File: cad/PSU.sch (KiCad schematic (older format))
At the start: 15 parts, among them J1 Input, J2 INA219 breakout, J3 Output, J4 WWG-A, J5 WWG-B, Q1 LM317T, U1 LM7805_TO220, U3 X9C103P

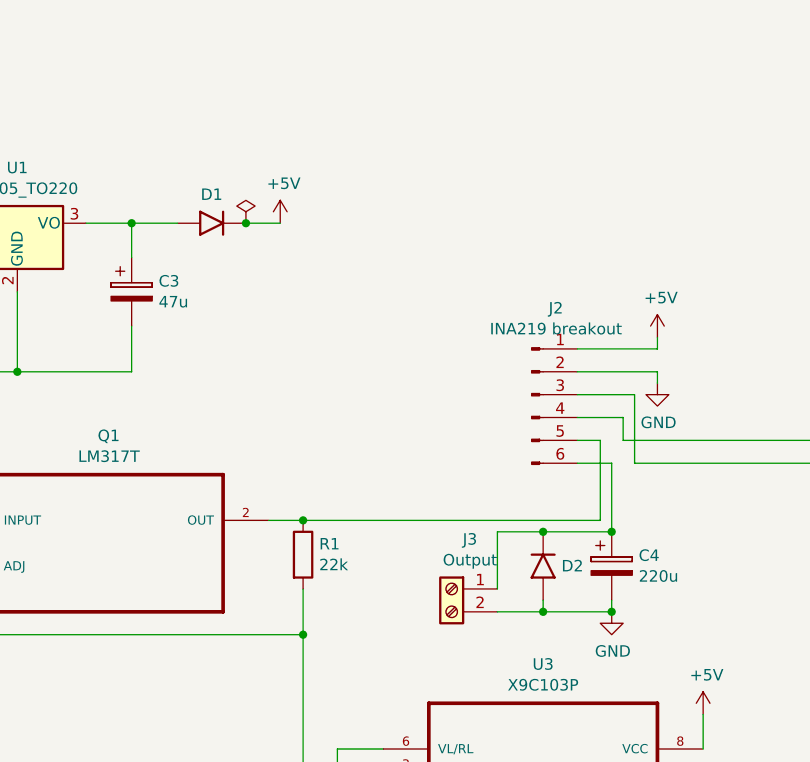
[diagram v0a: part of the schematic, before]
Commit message: first layout
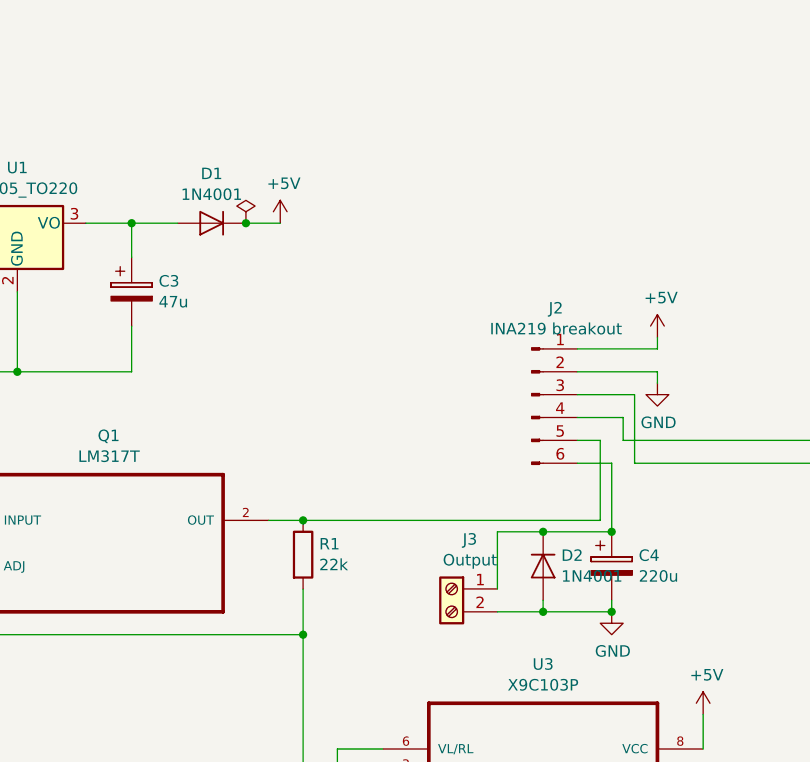
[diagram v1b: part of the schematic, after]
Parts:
- removed D1, D2: 1N4001, Diode_THT:D_A-405_P10.16mm_Horizontal, symbol 1N4001:1N4001
- added D1, D2: 1N4001, Diode_THT:D_DO-41_SOD81_P10.16mm_Horizontal, symbol Diode:1N4001
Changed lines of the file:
@@
 Wire Wire Line
 	7150 3200 7200 3200
-$Comp
-L 1N4001:1N4001 D1
-U 1 1 5CE165D2
-P 4200 2650
-F 0 "D1" H 4250 2775 50  0000 C CNN
-F 1 "1N4001" H 4200 2650 50  0001 L BNN
-F 2 "Diode_THT:D_A-405_P10.16mm_Horizontal" H 4200 2650 50  0001 L BNN
-F 3 "ON Semiconductor" H 4200 2650 50  0001 L BNN
-F 4 "None" H 4200 2650 50  0001 L BNN "Field4"
-F 5 "DO-41 ON Semiconductor" H 4200 2650 50  0001 L BNN "Field5"
-F 6 "Unavailable" H 4200 2650 50  0001 L BNN "Field6"
-F 7 "1N4001" H 4200 2650 50  0001 L BNN "Field7"
-F 8 "Diode, Standard, 1A, 50V" H 4200 2650 50  0001 L BNN "Field8"
-	1    4200 2650
-	1    0    0    -1
-$EndComp
 Wire Wire Line
 	3900 2650 4100 2650
@@
 Wire Wire Line
 	5500 4000 5500 4250
-Wire Wire Line
-	5500 4000 5700 4000
 Wire Wire Line
 	5500 4350 5700 4350
@@
 $EndComp
 Connection ~ 6000 4000
-$Comp
-L 1N4001:1N4001 D2
-U 1 1 5CE1E838
-P 5700 4200
-F 0 "D2" V 5750 4120 50  0000 R CNN
-F 1 "1N4001" H 5700 4200 50  0001 L BNN
-F 2 "Diode_THT:D_A-405_P10.16mm_Horizontal" H 5700 4200 50  0001 L BNN
-F 3 "ON Semiconductor" H 5700 4200 50  0001 L BNN
-F 4 "None" H 5700 4200 50  0001 L BNN "Field4"
-F 5 "DO-41 ON Semiconductor" H 5700 4200 50  0001 L BNN "Field5"
-F 6 "Unavailable" H 5700 4200 50  0001 L BNN "Field6"
-F 7 "1N4001" H 5700 4200 50  0001 L BNN "Field7"
-F 8 "Diode, Standard, 1A, 50V" H 5700 4200 50  0001 L BNN "Field8"
-	1    5700 4200
-	0    -1   -1   0
-$EndComp
-Connection ~ 5700 4000
-Wire Wire Line
-	5700 4000 6000 4000
 Wire Wire Line
 	6000 4300 6000 4350
@@
 	1    0    0    -1
 $EndComp
-Connection ~ 4400 2650
 Wire Wire Line
 	2500 4150 2650 4150
@@
 NoConn ~ 7200 3500
 NoConn ~ 5000 5050
+$Comp
+L Diode:1N4001 D1
+U 1 1 5CE7B69A
+P 4250 2650
+F 0 "D1" H 4250 2434 50  0000 C CNN
+F 1 "1N4001" H 4250 2525 50  0000 C CNN
+F 2 "Diode_THT:D_DO-41_SOD81_P10.16mm_Horizontal" H 4250 2475 50  0001 C CNN
+F 3 "http://www.vishay.com/docs/88503/1n4001.pdf" H 4250 2650 50  0001 C CNN
+	1    4250 2650
+	-1   0    0    1
+$EndComp
+Connection ~ 4400 2650
+Wire Wire Line
+	5500 4000 5700 4000
+$Comp
+L Diode:1N4001 D2
+U 1 1 5CE80A0F
+P 5700 4150
+F 0 "D2" V 5654 4229 50  0000 L CNN
+F 1 "1N4001" V 5745 4229 50  0000 L CNN
+F 2 "Diode_THT:D_DO-41_SOD81_P10.16mm_Horizontal" H 5700 3975 50  0001 C CNN
+F 3 "http://www.vishay.com/docs/88503/1n4001.pdf" H 5700 4150 50  0001 C CNN
+	1    5700 4150
+	0    1    1    0
+$EndComp
+Connection ~ 5700 4000
+Wire Wire Line
+	5700 4000 6000 4000
 $EndSCHEMATC
